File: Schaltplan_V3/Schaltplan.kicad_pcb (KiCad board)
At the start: 2 copper layers, 37.8 x 37.8 mm, 13 parts, among them IC1 STM32G031J6M6, J1 Conn_01x01, J2 Conn_01x04_Male, U1 HU2032-LF

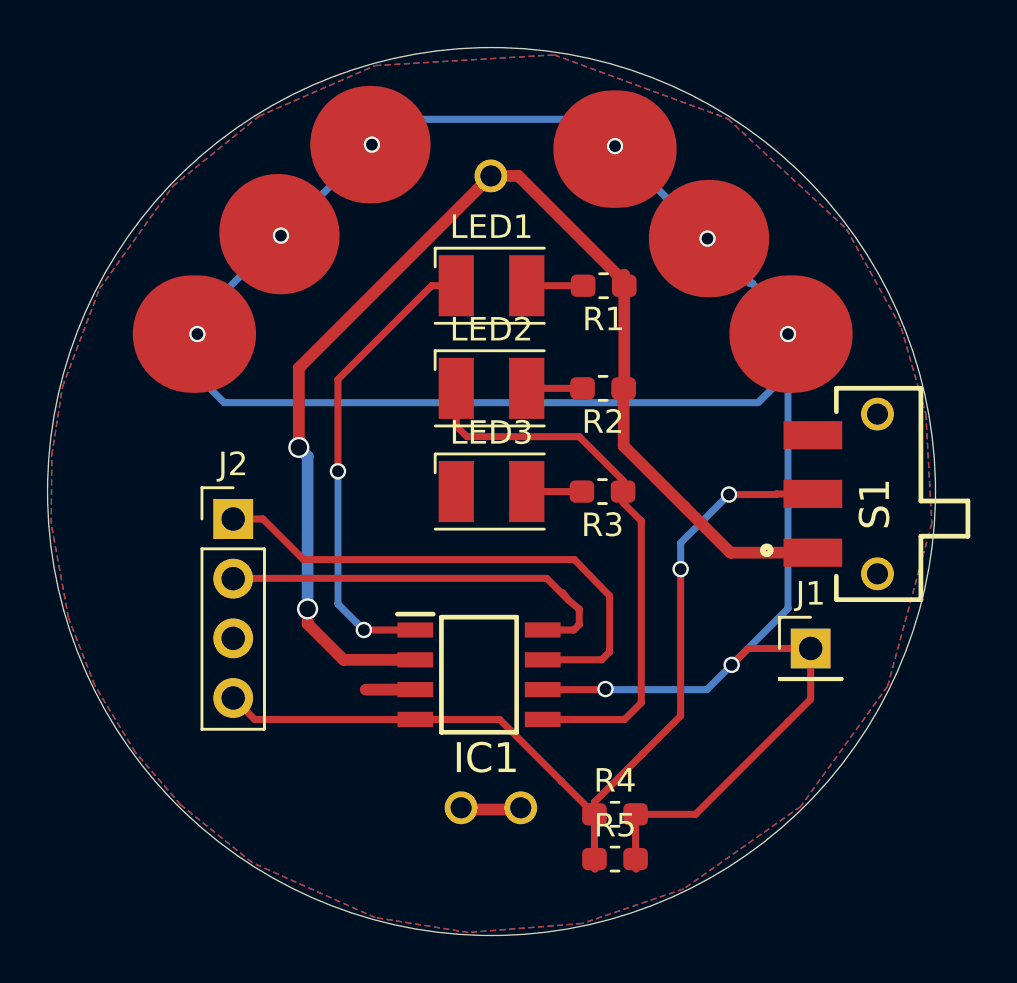
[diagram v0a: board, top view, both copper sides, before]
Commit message: mit Sensor, Platine fertig
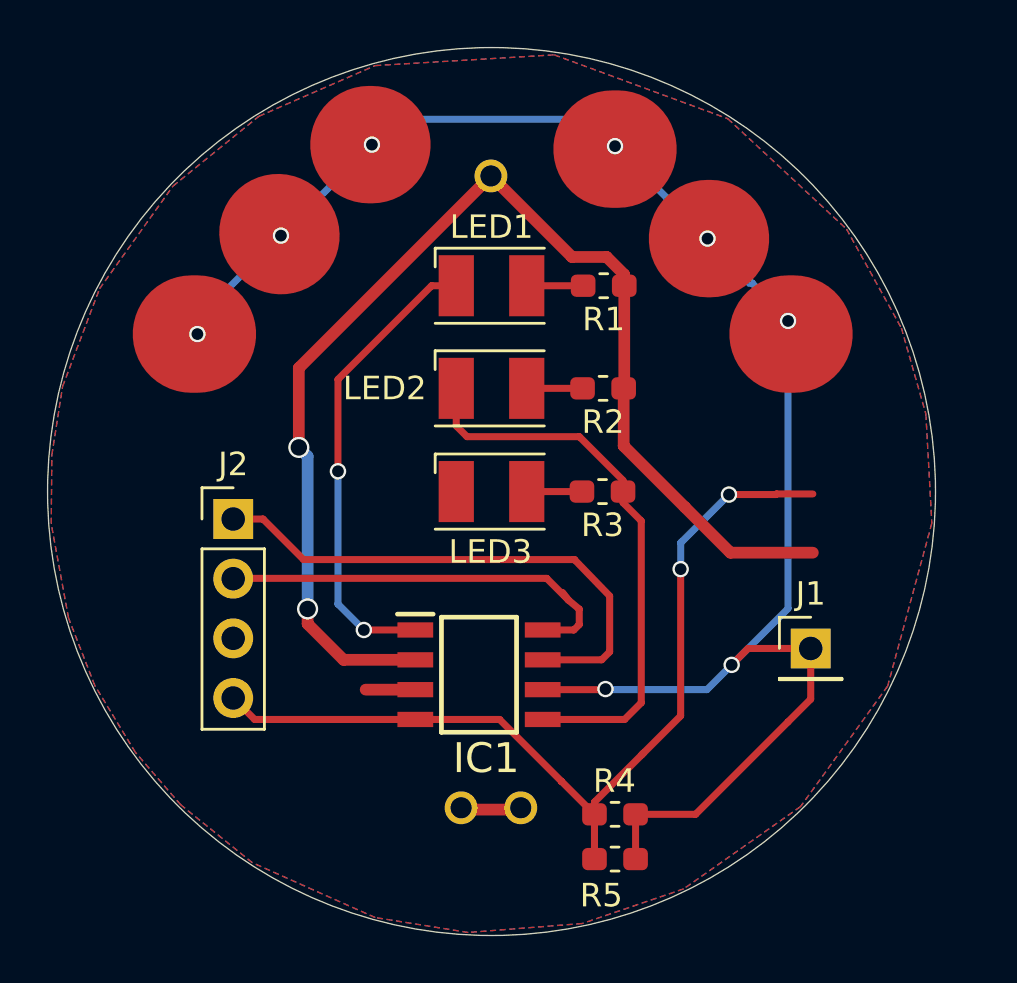
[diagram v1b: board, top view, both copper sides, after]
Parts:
- removed S1: JS102011SAQN, JS102011SAQN:JS102011SAQN
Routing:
- net PA12ReceivePin-kS: track 104.5 -> 76.5 mm
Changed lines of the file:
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@@
-(kicad_pcb (version 20171130) (host pcbnew "(5.1.6)-1")
+(kicad_pcb (version 20171130) (host pcbnew "(5.1.5)-3")
   (general
     (thickness 1.6)
     (drawings 1)
-    (tracks 137)
+    (tracks 130)
     (zones 0)
-    (modules 13)
-    (nets 13)
+    (modules 12)
+    (nets 12)
   )
   (page A4)
@@
     (aux_axis_origin 0 0)
     (grid_origin 156.845 111.379)
-    (visible_elements 7FFFFFFF)
+    (visible_elements 7FFDFF7F)
     (pcbplotparams
       (layerselection 0x010fc_ffffffff)
@@
   (net 10 "Net-(LED2-Pad2)")
   (net 11 "Net-(LED3-Pad2)")
-  (net 12 "Net-(S1-Pad3)")
   (net_class Default "Dies ist die voreingestellte Netzklasse."
     (clearance 0.3)
@@
     (add_net "Net-(LED2-Pad2)")
     (add_net "Net-(LED3-Pad2)")
-    (add_net "Net-(S1-Pad3)")
     (add_net PA8-LEDs)
     (add_net PB7-LEDs)
@@
     (tags "LED PLCC-2 SMD")
     (attr smd)
-    (fp_text reference LED2 (at 0 -2.5) (layer F.SilkS)
+    (fp_text reference LED2 (at -4.5452 0) (layer F.SilkS)
       (effects (font (size 1 1) (thickness 0.15)))
     )
@@
     (tags "LED PLCC-2 SMD")
     (attr smd)
-    (fp_text reference LED3 (at 0 -2.5) (layer F.SilkS)
+    (fp_text reference LED3 (at -0.0508 2.5654) (layer F.SilkS)
       (effects (font (size 1 1) (thickness 0.15)))
     )
@@
     (tags "resistor handsolder")
     (attr smd)
-    (fp_text reference R4 (at 0 -1.43) (layer F.SilkS)
+    (fp_text reference R4 (at -0.0254 -1.4224) (layer F.SilkS)
       (effects (font (size 1 1) (thickness 0.15)))
     )
@@
     (tags "resistor handsolder")
     (attr smd)
-    (fp_text reference R5 (at 0 -1.43) (layer F.SilkS)
+    (fp_text reference R5 (at -0.5842 1.5494) (layer F.SilkS)
       (effects (font (size 1 1) (thickness 0.15)))
     )
@@
     )
   )
-  (module JS102011SAQN:JS102011SAQN (layer F.Cu)
-    (at 158.9024 116.4082 90)
-    (descr JS102011SAQN)
-    (tags Switch)
-    (fp_text reference S1 (at -0.43 1.647 90) (layer F.SilkS)
-      (effects (font (size 1.27 1.27) (thickness 0.254)))
-    )
-    (fp_text value JS102011SAQN (at -0.43 1.647 90) (layer F.SilkS) hide
-      (effects (font (size 1.27 1.27) (thickness 0.254)))
-    )
-    (fp_circle (center -2.399 -2.96) (end -2.56315 -2.96) (layer F.SilkS) (width 0.254))
-    (fp_line (start 4.5 3.6) (end 4.5 0) (layer F.SilkS) (width 0.2))
-    (fp_line (start -0.3 3.6) (end 4.5 3.6) (layer F.SilkS) (width 0.2))
-    (fp_line (start -0.3 5.6) (end -0.3 3.6) (layer F.SilkS) (width 0.2))
-    (fp_line (start -1.8 5.6) (end -0.3 5.6) (layer F.SilkS) (width 0.2))
-    (fp_line (start -1.8 3.6) (end -1.8 5.6) (layer F.SilkS) (width 0.2))
-    (fp_line (start -4.5 3.6) (end -1.8 3.6) (layer F.SilkS) (width 0.2))
-    (fp_line (start -4.5 0) (end -4.5 3.6) (layer F.SilkS) (width 0.2))
-    (fp_line (start -0.3 5.6) (end -0.3 3.6) (layer Dwgs.User) (width 0.2))
-    (fp_line (start -1.8 5.6) (end -0.3 5.6) (layer Dwgs.User) (width 0.2))
-    (fp_line (start -1.8 3.6) (end -1.8 5.6) (layer Dwgs.User) (width 0.2))
-    (fp_line (start -4.5 0) (end -3.5 0) (layer F.SilkS) (width 0.2))
-    (fp_line (start 4.5 0) (end 3.5 0) (layer F.SilkS) (width 0.2))
-    (fp_line (start -4.5 3.6) (end -4.5 0) (layer Dwgs.User) (width 0.2))
-    (fp_line (start 4.5 3.6) (end -4.5 3.6) (layer Dwgs.User) (width 0.2))
-    (fp_line (start 4.5 0) (end 4.5 3.6) (layer Dwgs.User) (width 0.2))
-    (fp_line (start -4.5 0) (end 4.5 0) (layer Dwgs.User) (width 0.2))
-    (pad 1 smd rect (at -2.5 -1 90) (size 1.2 2.5) (layers F.Cu F.Paste F.Mask)
-      (net 2 +3V3))
-    (pad 2 smd rect (at 0 -1 90) (size 1.2 2.5) (layers F.Cu F.Paste F.Mask)
-      (net 4 Conn-RST))
-    (pad 3 smd rect (at 2.5 -1 90) (size 1.2 2.5) (layers F.Cu F.Paste F.Mask)
-      (net 12 "Net-(S1-Pad3)"))
-    (pad 4 thru_hole circle (at -3.4 1.75 180) (size 1.4 1.4) (drill 0.9) (layers *.Cu *.Mask F.SilkS))
-    (pad 5 thru_hole circle (at 3.4 1.75 180) (size 1.4 1.4) (drill 0.9) (layers *.Cu *.Mask F.SilkS))
-  )
   (gr_circle (center 144.2212 116.304918) (end 161.417 108.458) (layer Edge.Cuts) (width 0.05))
   (via (at 138.7856 122.1994) (size 0.7) (drill 0.5) (layers F.Cu B.Cu) (net 1))
@@
   (segment (start 141.6712 107.5436) (end 137.683056 111.531744) (width 0.3) (layer F.Cu) (net 1))
   (segment (start 137.683056 111.531744) (end 137.683056 115.4416) (width 0.3) (layer F.Cu) (net 1))
-  (segment (start 149.8714 107.0686) (end 149.8714 107.5436) (width 0.5) (layer F.Cu) (net 2))
   (segment (start 136.390199 121.302599) (end 136.390199 121.302599) (width 0.5) (layer B.Cu) (net 2))
   (via (at 136.390199 121.302599) (size 0.9) (drill 0.7) (layers F.Cu B.Cu) (net 2))
@@
   (via (at 136.017002 114.426998) (size 0.9) (drill 0.7) (layers F.Cu B.Cu) (net 2))
   (segment (start 144.1958 102.8686) (end 136.017002 111.047398) (width 0.5) (layer F.Cu) (net 2))
-  (segment (start 145.367952 102.8686) (end 144.1958 102.8686) (width 0.5) (layer F.Cu) (net 2))
-  (segment (start 149.8714 107.372048) (end 145.367952 102.8686) (width 0.5) (layer F.Cu) (net 2))
-  (segment (start 149.8714 107.5436) (end 149.8714 107.372048) (width 0.5) (layer F.Cu) (net 2))
+  (segment (start 149.8714 107.0686) (end 149.8714 107.5436) (width 0.5) (layer F.Cu) (net 2))
+  (segment (start 149.12139 106.31859) (end 149.8714 107.0686) (width 0.5) (layer F.Cu) (net 2))
+  (segment (start 147.64579 106.31859) (end 149.12139 106.31859) (width 0.5) (layer F.Cu) (net 2))
+  (segment (start 144.1958 102.8686) (end 147.64579 106.31859) (width 0.5) (layer F.Cu) (net 2))
   (segment (start 145.3896 129.8448) (end 142.8496 129.8448) (width 0.5) (layer F.Cu) (net 3) (status 30))
   (segment (start 138.8618 124.7394) (end 140.9758 124.7394) (width 0.5) (layer F.Cu) (net 3))
-  (segment (start 148.5786 132.334) (end 148.6294 132.3848) (width 0.3) (layer F.Cu) (net 4))
   (segment (start 150.6182 127.508) (end 150.622 127.508) (width 0.3) (layer F.Cu) (net 4))
   (segment (start 140.9758 126.0094) (end 144.5654 126.0094) (width 0.3) (layer F.Cu) (net 4))
@@
   (segment (start 155.1432 122.9868) (end 154.4447 123.6853) (width 0.3) (layer F.Cu) (net 8))
   (segment (start 157.8102 122.9868) (end 155.1432 122.9868) (width 0.3) (layer F.Cu) (net 8))
-  (segment (start 150.3286 132.334) (end 150.3794 132.3848) (width 0.3) (layer F.Cu) (net 8))
   (segment (start 154.4447 123.6853) (end 156.845 121.285) (width 0.3) (layer B.Cu) (net 8))
   (segment (start 148.336 100.457) (end 148.336 100.457) (width 0.3) (layer B.Cu) (net 8))
@@
   (segment (start 156.845 108.966) (end 155.321 107.442) (width 0.3) (layer B.Cu) (net 8))
   (segment (start 156.845 108.966) (end 156.845 108.966) (width 0.3) (layer B.Cu) (net 8))
-  (via (at 156.845 109.601) (size 0.7) (drill 0.5) (layers F.Cu B.Cu) (net 8))
+  (via (at 156.845 109.0422) (size 0.7) (drill 0.5) (layers F.Cu B.Cu) (net 8))
   (via (at 149.479 101.6) (size 0.7) (drill 0.5) (layers F.Cu B.Cu) (net 8))
   (segment (start 150.3286 130.0226) (end 150.6474 130.0226) (width 0.3) (layer F.Cu) (net 8))
@@
   (segment (start 156.845 126.111) (end 157.8102 125.1458) (width 0.3) (layer F.Cu) (net 8))
   (segment (start 150.354 130.048) (end 150.354 131.953) (width 0.3) (layer F.Cu) (net 8))
-  (segment (start 156.845 111.252) (end 156.845 108.966) (width 0.3) (layer B.Cu) (net 8))
-  (segment (start 156.845 121.285) (end 156.845 111.252) (width 0.3) (layer B.Cu) (net 8))
   (segment (start 140.589 100.457) (end 140.589 100.457) (width 0.3) (layer B.Cu) (net 8))
-  (segment (start 155.575 112.522) (end 156.845 111.252) (width 0.3) (layer B.Cu) (net 8))
-  (segment (start 132.969 112.522) (end 155.575 112.522) (width 0.3) (layer B.Cu) (net 8))
-  (segment (start 132.842 112.522) (end 132.969 112.522) (width 0.3) (layer B.Cu) (net 8))
-  (segment (start 131.699 111.379) (end 132.842 112.522) (width 0.3) (layer B.Cu) (net 8))
   (segment (start 131.699 109.347) (end 131.699 109.601) (width 0.3) (layer B.Cu) (net 8))
   (segment (start 149.5425 101.6635) (end 148.336 100.457) (width 0.3) (layer B.Cu) (net 8))
-  (segment (start 131.699 109.601) (end 131.699 111.379) (width 0.3) (layer B.Cu) (net 8))
   (via (at 131.699 109.601) (size 0.7) (drill 0.5) (layers F.Cu B.Cu) (net 8))
   (segment (start 148.336 100.457) (end 140.208 100.457) (width 0.3) (layer B.Cu) (net 8))
@@
   (segment (start 149.606 101.727) (end 149.352 101.727) (width 5) (layer F.Cu) (net 8))
   (segment (start 139.0015 101.5365) (end 139.1285 101.5365) (width 5) (layer F.Cu) (net 8))
+  (segment (start 156.845 108.966) (end 156.845 109.601) (width 0.3) (layer B.Cu) (net 8))
+  (segment (start 156.845 121.285) (end 156.845 109.601) (width 0.3) (layer B.Cu) (net 8))
   (segment (start 148.1214 107.5436) (end 145.7212 107.5436) (width 0.3) (layer F.Cu) (net 9))
   (segment (start 148.096 111.9124) (end 145.7198 111.9124) (width 0.3) (layer F.Cu) (net 10))
